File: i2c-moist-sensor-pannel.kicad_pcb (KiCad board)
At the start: 2 copper layers, 100 x 150 mm, 140 parts, among them IC1 ATTINY441-SSU, P1 CONN_02X03, X1 16MHz

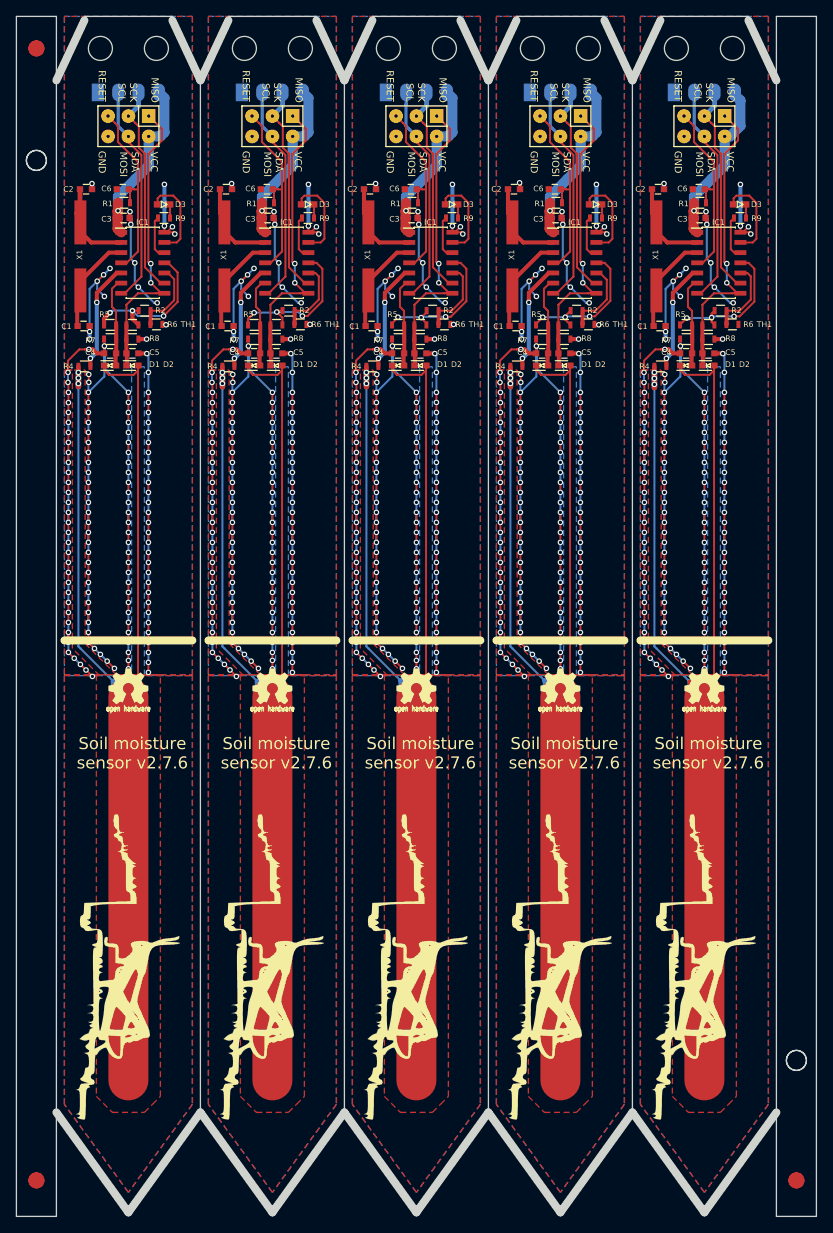
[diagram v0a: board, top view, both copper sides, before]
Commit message: Shuffle stuff around
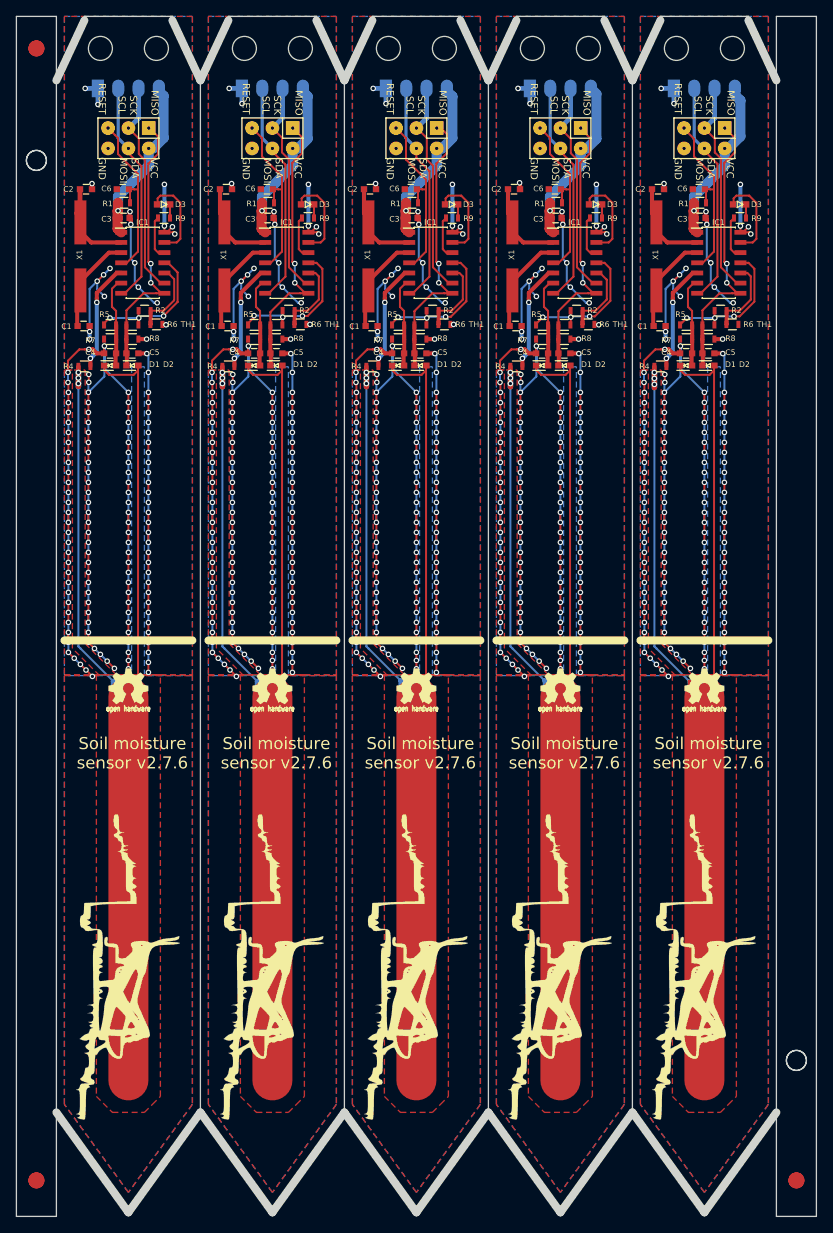
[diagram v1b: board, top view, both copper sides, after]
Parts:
- removed the P1 at (94.0, 35.7)
- removed the P1 at (112.0, 35.7)
- removed the P1 at (130.0, 35.7)
- removed the P1 at (148.0, 35.7)
- removed the P1 at (166.0, 35.7)
- removed the REF** at (177.5, 167.5) (x2)
- removed the REF** at (82.5, 40.0) (x2)
- removed the REF** at (82.5, 167.5) (x2)
- removed the REF** at (82.5, 26.0) (x2)
- removed the REF** at (177.5, 152.5) (x2)
- added P1: CONN_02X03, Pin_Headers:Pin_Header_Straight_2x03, F.Cu at (148.0, 37.2)
- added P1: CONN_02X03, Pin_Headers:Pin_Header_Straight_2x03, F.Cu at (130.0, 37.2)
- added P1: CONN_02X03, Pin_Headers:Pin_Header_Straight_2x03, F.Cu at (94.0, 37.2)
- added P1: CONN_02X03, Pin_Headers:Pin_Header_Straight_2x03, F.Cu at (112.0, 37.2)
- added P1: CONN_02X03, Pin_Headers:Pin_Header_Straight_2x03, F.Cu at (166.0, 37.2)
- added REF** (x2): Fiducial_Modern_CopperTop, Fiducials:Fiducial_Modern_CopperTop, F.Cu at (177.5, 167.5)
- added REF** (x2): MountingHole_2-5mm, Mounting_Holes:MountingHole_2-5mm, F.Cu at (82.5, 40.0)
- added REF** (x2): Fiducial_Modern_CopperTop, Fiducials:Fiducial_Modern_CopperTop, F.Cu at (82.5, 167.5)
- added REF** (x2): Fiducial_Modern_CopperTop, Fiducials:Fiducial_Modern_CopperTop, F.Cu at (82.5, 26.0)
- added REF** (x2): MountingHole_2-5mm, Mounting_Holes:MountingHole_2-5mm, F.Cu at (177.5, 152.5)
- moved PIN_SOCKET_4 0.50 mm to (94.0, 31.0)
- moved PIN_SOCKET_4 0.50 mm to (112.0, 31.0)
- moved PIN_SOCKET_4 0.50 mm to (130.0, 31.0)
- moved PIN_SOCKET_4 0.50 mm to (148.0, 31.0)
- moved PIN_SOCKET_4 0.50 mm to (166.0, 31.0)
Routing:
- net GND: track 1120.3 -> 1137.7 mm, vias 724 -> 734
- net /MISO/SENSE_HIGH: track 190.6 -> 176.7 mm
- net /RESET: track 120.4 -> 113.3 mm
- net /POWER: track 97.4 -> 93.7 mm
- net VCC: track 111.8 -> 113.6 mm
